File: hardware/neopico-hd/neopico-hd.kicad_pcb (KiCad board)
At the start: 2 copper layers, 70.1 x 72.2 mm, 24 parts, among them J1 HDMI_A, J2 Conn_02x05_Top_Bottom, J3 Audio, J4 Audio, J5 AUX, J6 Conn_01x02_Pin, U1 A_BUFF, U2 V_BUFF, U3 RG_LVS, U4 GB_LVS, U5 AV_LVS

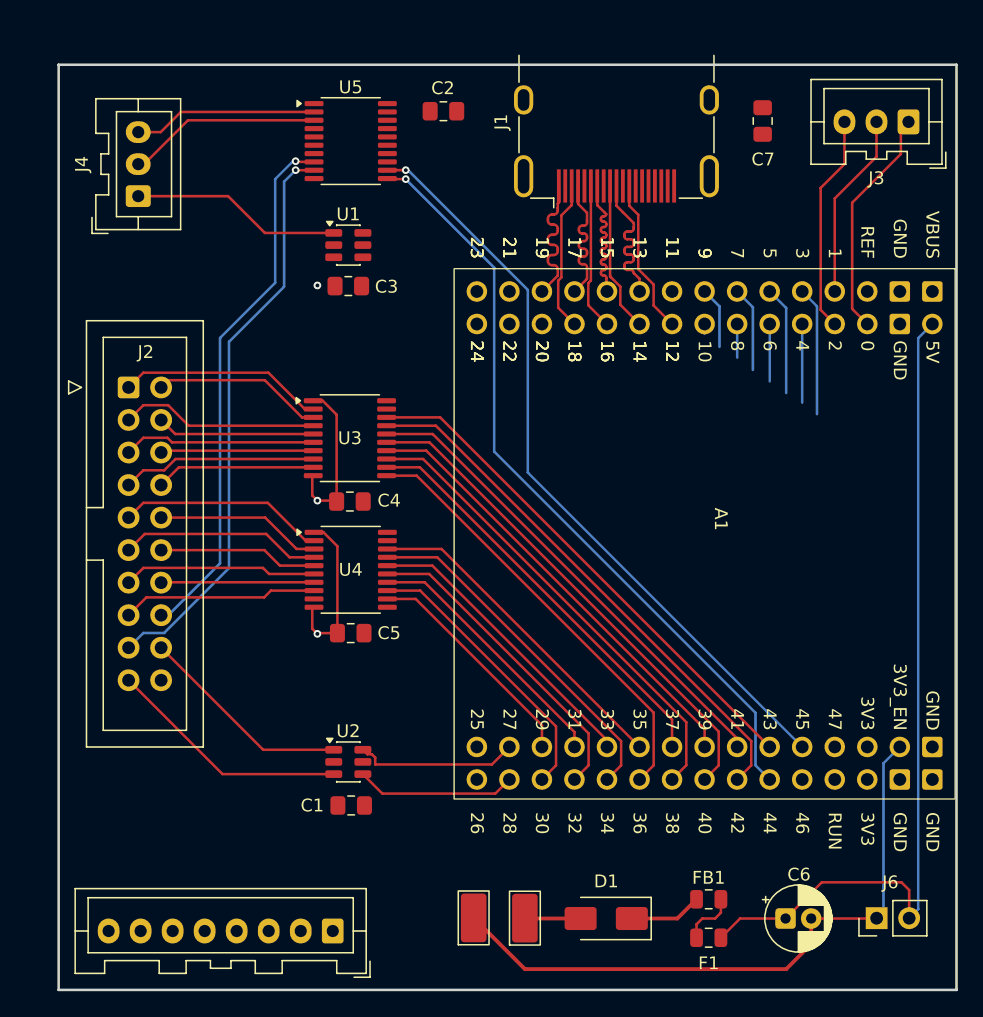
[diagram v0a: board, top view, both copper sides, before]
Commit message: V1 PCB
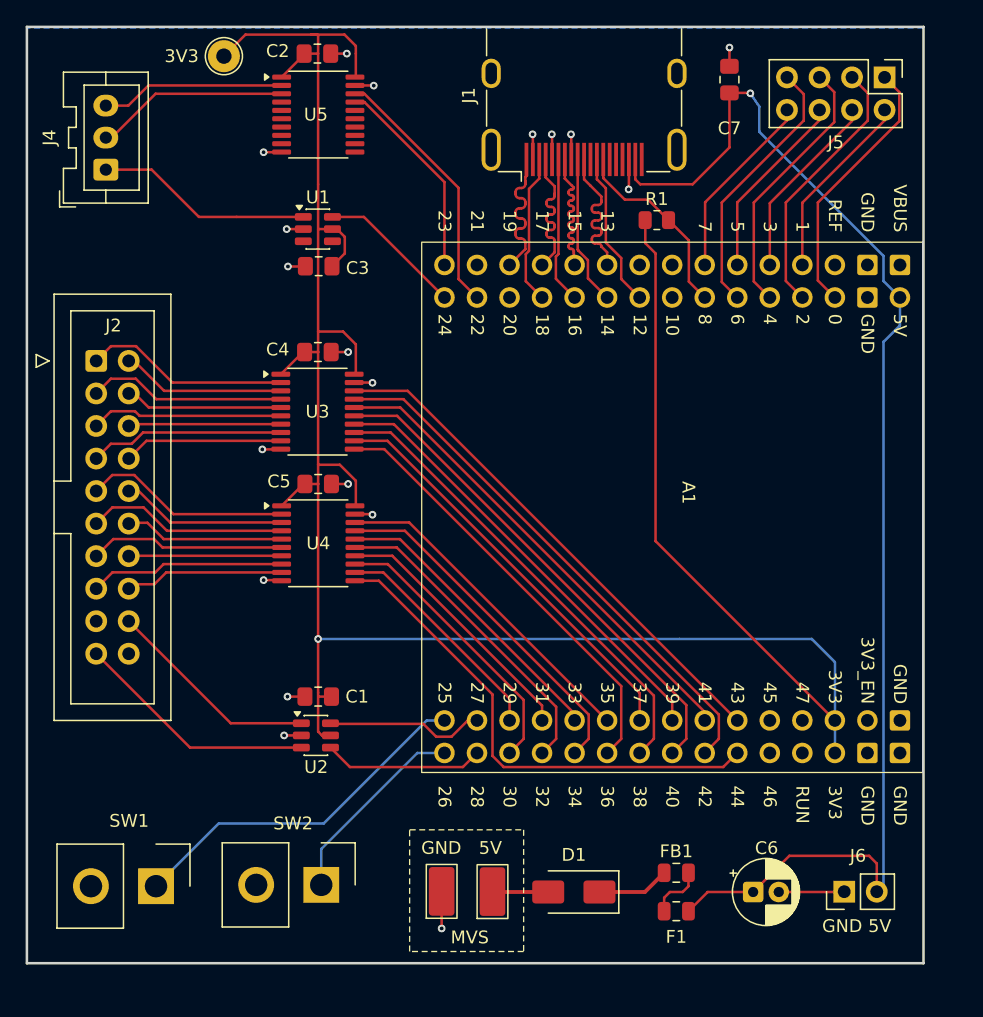
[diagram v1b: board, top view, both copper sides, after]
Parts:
- removed J3: Audio, Connector_JST:JST_XA_B03B-XASK-1_1x03_P2.50mm_Vertical
- added 3V3: TestPoint_THTPad_D2.5mm_Drill1.2mm, TestPoint:TestPoint_THTPad_D2.5mm_Drill1.2mm, F.Cu at (130.9, 37.3)
- added R1: 27K, Resistor_SMD:R_0805_2012Metric, F.Cu at (164.7, 50.1)
- added SW1: MENU, Connector_Samtec_HPM_THT:Samtec_HPM-02-01-x-S_Straight_1x02_Pitch5.08mm, F.Cu at (125.6, 102.1)
- added SW2: BACK, Connector_Samtec_HPM_THT:Samtec_HPM-02-01-x-S_Straight_1x02_Pitch5.08mm, F.Cu at (138.5, 102.0)
- J5: footprint Connector_JST:JST_XA_B08B-XASK-1_1x08_P2.50mm_Vertical -> Connector_PinHeader_2.54mm:PinHeader_2x04_P2.54mm_Vertical
- moved J5 79.4 mm to (182.5, 39.0), turned to -90 degrees
- moved C4 11.9 mm to (138.2, 60.4), turned to 0 degrees
- moved C5 11.9 mm to (138.3, 70.7), turned to 0 degrees
- moved C2 10.8 mm to (138.2, 37.1), turned to 0 degrees
- moved C1 8.88 mm to (138.3, 87.3), turned to 180 degrees
- moved C7 4.14 mm to (170.4, 39.1)
- moved A1 3.27 mm to (165.9, 71.4)
- moved U2 3.27 mm to (138.1, 90.3)
- moved U4 3.27 mm to (138.3, 75.3)
- moved J1 3.27 mm to (159.0, 42.1)
- moved J4 3.27 mm to (121.7, 46.2)
- moved U5 3.27 mm to (138.3, 41.9)
- moved C6 3.27 mm to (172.2, 102.6)
- moved D1 3.27 mm to (158.2, 102.6)
- moved F1 3.27 mm to (166.2, 104.1)
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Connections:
- A1 pad 14: Net-(A1-GPIO8) -> CEC_PICO
- A1 pad 15: Net-(A1-GPIO9) -> unconnected-(A1-GPIO9-Pad15)
- A1 pad 16: Net-(A1-GPIO10) -> unconnected-(A1-GPIO10-Pad16)
- A1 pad 31: unconnected-(A1-GPIO25-Pad31) -> SW_MENU
- A1 pad 32: unconnected-(A1-GPIO26-Pad32) -> SW_BACK
- A1 pad 51: DARK -> unconnected-(A1-GPIO45-Pad51)
- A1 pad 54: (no net) -> unconnected-(A1-RUN-Pad54)
- A1 pad 57: GND -> unconnected-(A1-EN-Pad57)
- A1 pad 58: (no net) -> GND
- J1 pad 13: unconnected-(J1-CEC-Pad13) -> CEC_PICO
- J1 pad 2: unconnected-(J1-D2S-Pad2) -> GND
- J1 pad 5: unconnected-(J1-D1S-Pad5) -> GND
- J1 pad 8: unconnected-(J1-D0S-Pad8) -> GND
- J1 pad SH: unconnected-(J1-PadSH)_3 -> GND
- J2 pad 17: MVS_DARK -> unconnected-(J2-Pin_17-Pad17)
- J5 pad 1: Net-(A1-GPIO3) -> Net-(A1-GPIO0)
- J5 pad 2: Net-(A1-GPIO4) -> Net-(A1-GPIO1)
- J5 pad 3: Net-(A1-GPIO5) -> Net-(A1-GPIO2)
- J5 pad 4: Net-(A1-GPIO6) -> Net-(A1-GPIO3)
- J5 pad 5: Net-(A1-GPIO7) -> Net-(A1-GPIO4)
- J5 pad 6: Net-(A1-GPIO8) -> Net-(A1-GPIO5)
- J5 pad 7: Net-(A1-GPIO9) -> Net-(A1-GPIO6)
- J5 pad 8: Net-(A1-GPIO10) -> Net-(A1-GPIO7)
- U3 pad 1: GND -> +3V3
- U3 pad 19: +3V3 -> GND
- U4 pad 1: GND -> +3V3
- U4 pad 11: unconnected-(U4-B8-Pad11) -> SHD
- U4 pad 19: +3V3 -> GND
- U4 pad 9: unconnected-(U4-A8-Pad9) -> MVS_SHD
- U5 pad 1: GND -> +3V3
- U5 pad 11: DARK -> unconnected-(U5-B8-Pad11)
- U5 pad 12: SHD -> unconnected-(U5-B7-Pad12)
- U5 pad 19: +3V3 -> GND
- U5 pad 8: MVS_SHD -> unconnected-(U5-A7-Pad8)
- U5 pad 9: MVS_DARK -> unconnected-(U5-A8-Pad9)
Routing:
- net +3V3: track 0.00 -> 191.3 mm, vias 0 -> 1
- net DARK: track 59.4 -> 0.00 mm, vias 1 -> 0
- net MVS_DARK: track 45.1 -> 0.00 mm, vias 1 -> 0
- net GND: track 75.7 -> 36.3 mm, vias 2 -> 19
- net +5V: track 66.1 -> 102.9 mm, vias 0 -> 1
- net MVS_SHD: track 41.7 -> 12.5 mm, vias 1 -> 0
- net SW_MENU: track 0.00 -> 29.1 mm
- net SHD: track 60.1 -> 39.1 mm, vias 1 -> 0
- net DAT: track 0.00 -> 20.3 mm
- net Net-(A1-GPIO6): track 4.48 -> 20.9 mm
- net WS: track 0.00 -> 16.0 mm
- net SW_BACK: track 0.00 -> 15.5 mm
- net CEC_PICO: track 0.00 -> 15.1 mm
- net Net-(A1-GPIO4): track 6.13 -> 20.8 mm
- net BCK: track 0.00 -> 11.4 mm
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- added copper zone on B.Cu, net GND
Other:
- board size 70.1 x 72.2 mm -> 70 x 73.1 mm
- board text added: "5V"
- board text added: "GND"
- board text added: "MVS"
- board text removed: "11"
- board text removed: "12"
- board text removed: "13"
- board text removed: "14"
- board text removed: "15"
- board text removed: "16"
- board text removed: "17"
- board text removed: "18"
- board text removed: "19"
- board text removed: "20"
- board text removed: "21"
- board text removed: "22"
- board text removed: "23"
- board text removed: "24"
- board text removed: "9"
